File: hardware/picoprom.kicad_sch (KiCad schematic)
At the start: 15 parts, among them U1 Pico, U2 TXB0108PWR, U3 28C256

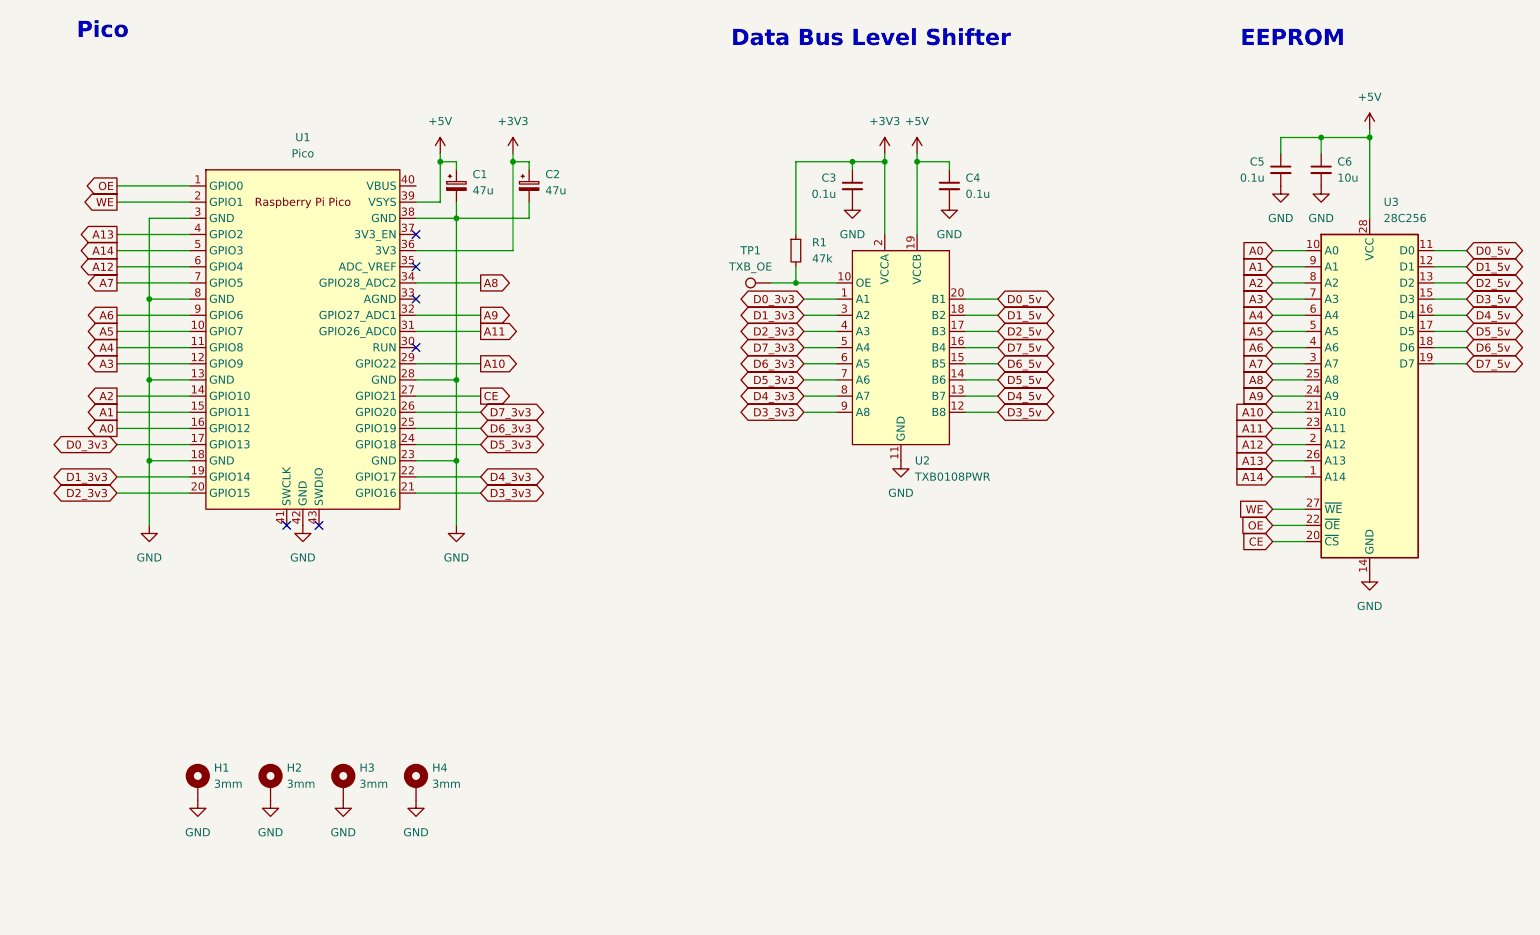
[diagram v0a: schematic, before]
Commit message: Final edits to hardware for Rev0.
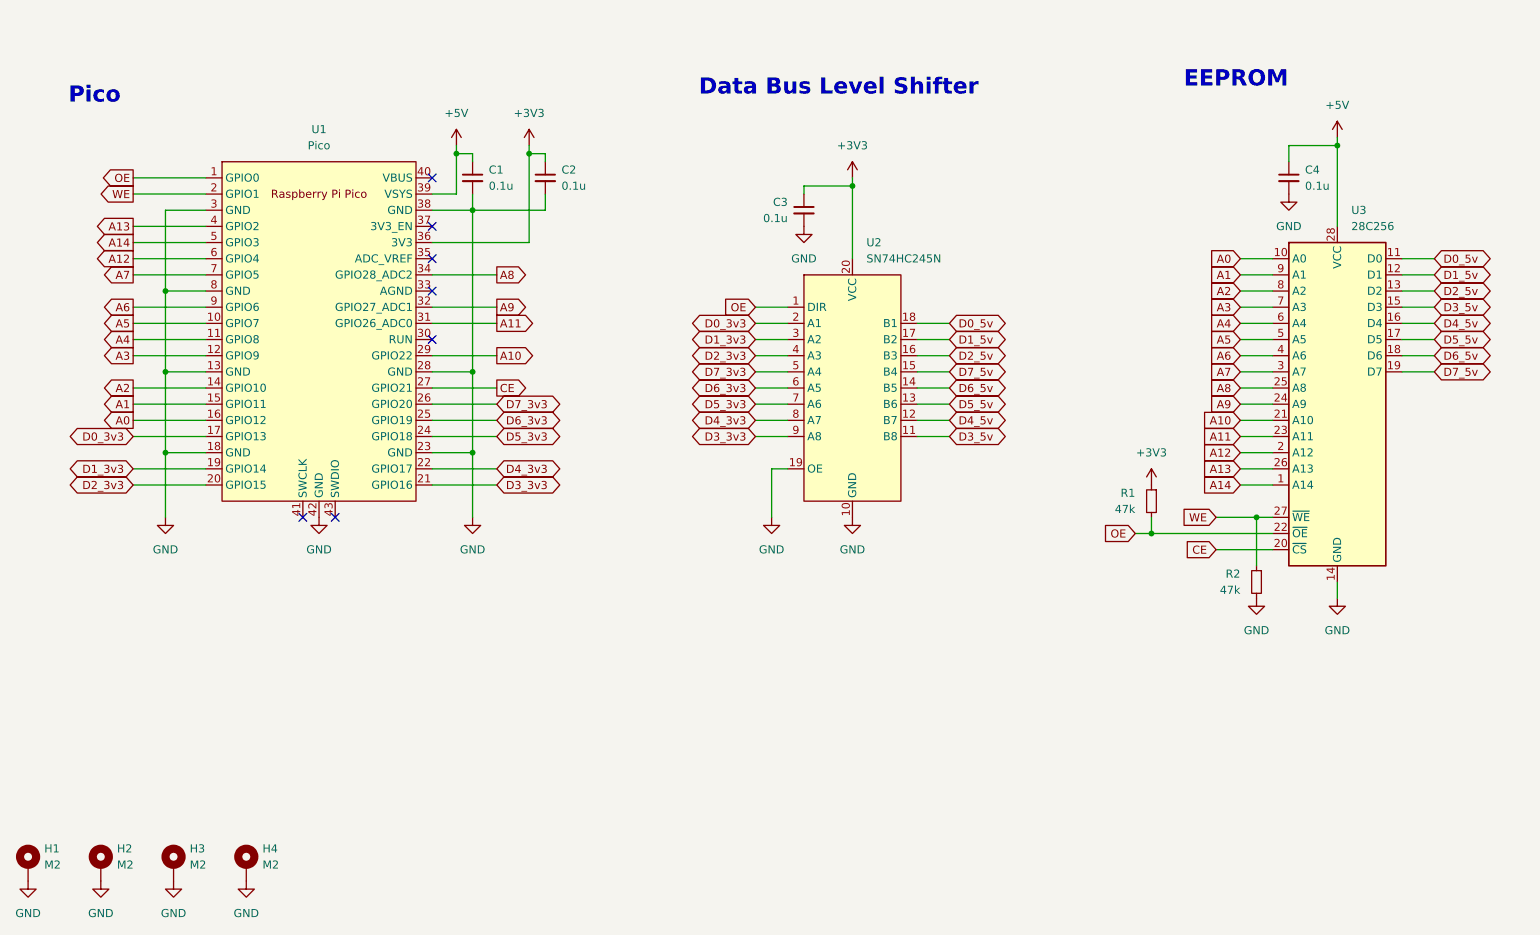
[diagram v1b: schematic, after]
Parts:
- removed C1, C2: 47u, Capacitor_SMD:CP_Elec_6.3x5.8, symbol Device:C_Polarized_Small
- removed C4, C5: 0.1u, Capacitor_SMD:C_0805_2012Metric_Pad1.18x1.45mm_HandSolder, symbol Device:C_Small
- removed TP1: TXB_OE, TestPoint:TestPoint_Pad_D2.0mm, symbol Connector:TestPoint
- removed U2: TXB0108PWR, Package_SO:TSSOP-20_4.4x6.5mm_P0.65mm, symbol picoprom:TXB0108PWR
- added C1, C2: 0.1u, Capacitor_THT:C_Rect_L4.0mm_W2.5mm_P2.50mm, symbol Device:C_Small
- added R2: 47k, Resistor_THT:R_Axial_DIN0204_L3.6mm_D1.6mm_P5.08mm_Horizontal, symbol Device:R_Small
- added U2: SN74HC245N, Package_DIP:DIP-20_W7.62mm_Socket_LongPads, symbol picoprom:SN74HC245N
- C3: footprint Capacitor_SMD:C_0805_2012Metric_Pad1.18x1.45mm_HandSolder -> Capacitor_THT:C_Rect_L4.0mm_W2.5mm_P2.50mm
- C4: renamed from C6; value 10u -> 0.1u; footprint Capacitor_SMD:C_0805_2012Metric_Pad1.18x1.45mm_HandSolder -> Capacitor_THT:C_Rect_L4.0mm_W2.5mm_P2.50mm
- H1, H2, H3, H4: value 3mm -> M2; footprint MountingHole:MountingHole_3mm_Pad -> MountingHole:MountingHole_2.2mm_M2_Pad
- R1: footprint Resistor_SMD:R_0805_2012Metric_Pad1.20x1.40mm_HandSolder -> Resistor_THT:R_Axial_DIN0204_L3.6mm_D1.6mm_P5.08mm_Horizontal
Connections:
- net +3V3: now also C2.1, U2.20 (VCC)
- net +5V: now also C1.1
- net D0_3v3: now also U2.2 (A1)
- net D0_5v: now also U2.18 (B1)
- net D1_3v3: now also U2.3 (A2)
- net D1_5v: now also U2.17 (B2)
- net D2_3v3: now also U2.4 (A3)
- net D2_5v: now also U2.16 (B3)
- net D3_3v3: now also U2.9 (A8)
- net D3_5v: now also U2.11 (B8)
- net D4_3v3: now also U2.8 (A7)
- net D4_5v: now also U2.12 (B7)
- net D5_3v3: now also U2.7 (A6)
- net D5_5v: now also U2.13 (B6)
- net D6_3v3: now also U2.6 (A5)
- net D6_5v: now also U2.14 (B5)
- net D7_3v3: now also U2.5 (A4)
- net D7_5v: now also U2.15 (B4)
- net GND: now also C1.2, C2.2, R2.2, U2.10 (GND), U2.19 (OE)
- net OE: now also R1.2, U2.1 (DIR)
- net WE: now also R2.1
- no-connect marks 6 -> 7
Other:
- moved on the sheet: C4, H1, H2, H3, H4, U1, U3
